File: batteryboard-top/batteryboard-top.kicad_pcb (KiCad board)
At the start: 2 copper layers, 46.8 x 46.8 mm, 7 parts, among them J1 FLE-105-01-G-DV-A, J2 FLE-105-01-G-DV-A

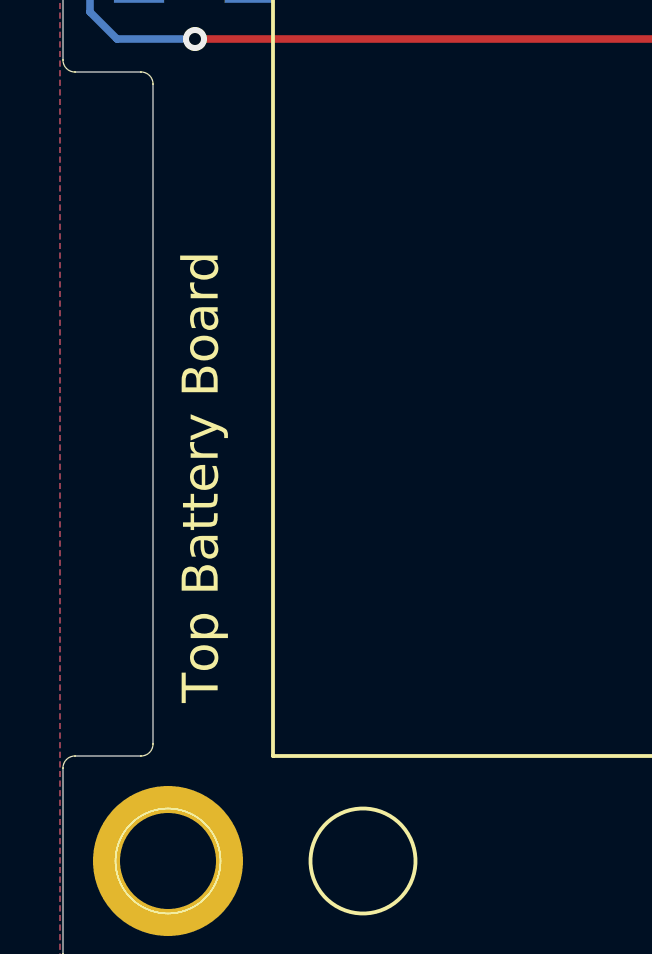
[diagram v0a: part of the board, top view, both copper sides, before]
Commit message: Export New Gerbers
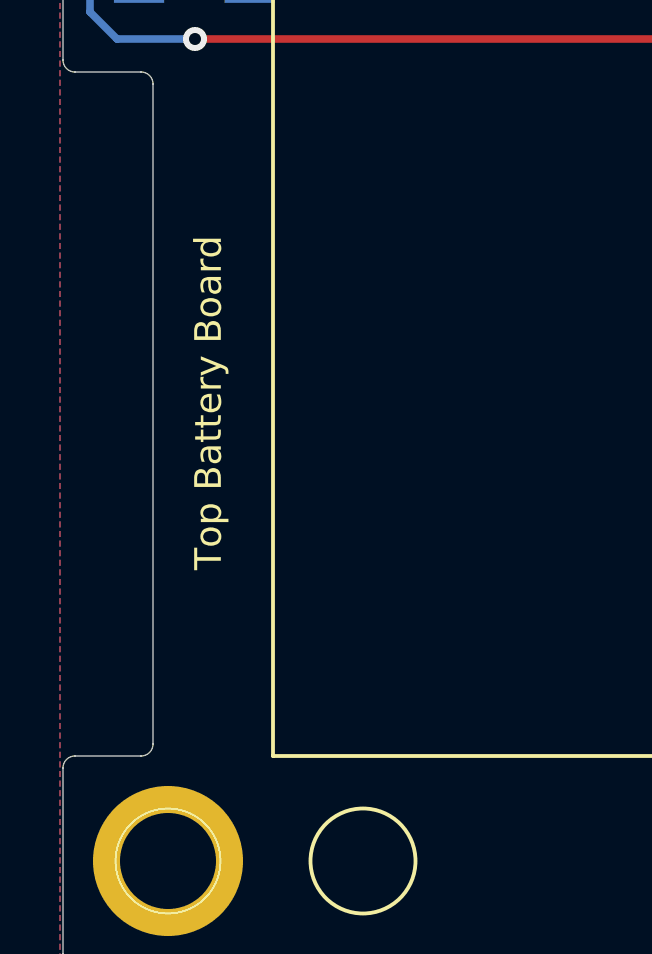
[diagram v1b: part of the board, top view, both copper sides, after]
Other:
- board text added: "06-JUL-22"
- board text removed: "29-JUN-22"
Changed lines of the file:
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@@
       (drillshape 0)
       (scaleselection 1)
-      (outputdirectory "../gerbers/batteryboard-top (06-13-22)/")
+      (outputdirectory "../gerbers/batteryboard-top (07-06-22)/")
     )
   )
@@
   (gr_arc (start 171.199988 112.900003) (mid 170.917151 112.782841) (end 170.799988 112.500004) (layer "Edge.Cuts") (width 0.0254))
   (gr_line (start 127.399999 112.900003) (end 129.6 112.899993) (layer "Edge.Cuts") (width 0.0254))
-  (gr_text "Top Battery Board" (at 131.6 103.6 90) (layer "F.SilkS")
-    (effects (font (size 1.2 1.2) (thickness 0.2)))
+  (gr_text "Top Battery Board" (at 131.850003 101.124995 90) (layer "F.SilkS")
+    (effects (font (size 0.889 0.889) (thickness 0.127)))
   )
-  (gr_text "29-JUN-22" (at 152.318796 75.512422) (layer "F.Mask")
+  (gr_text "06-JUL-22" (at 152.318796 75.512422) (layer "F.Mask")
     (effects (font (size 0.635 0.635) (thickness 0.1524)) (justify right))
   )
